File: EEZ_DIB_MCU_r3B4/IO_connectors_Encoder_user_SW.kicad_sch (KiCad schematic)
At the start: 39 parts, among them IC1 TPD4E001DRLR, IC2 74AUP1G74DC.125, IC3 CD74HC4050PWR, SW1 TL1100CF160Q, SW2 PEC16-2215F-S0024, X1 DS1024-2*20R0, X2 DS1013-16SSIB1, X3 691322110005

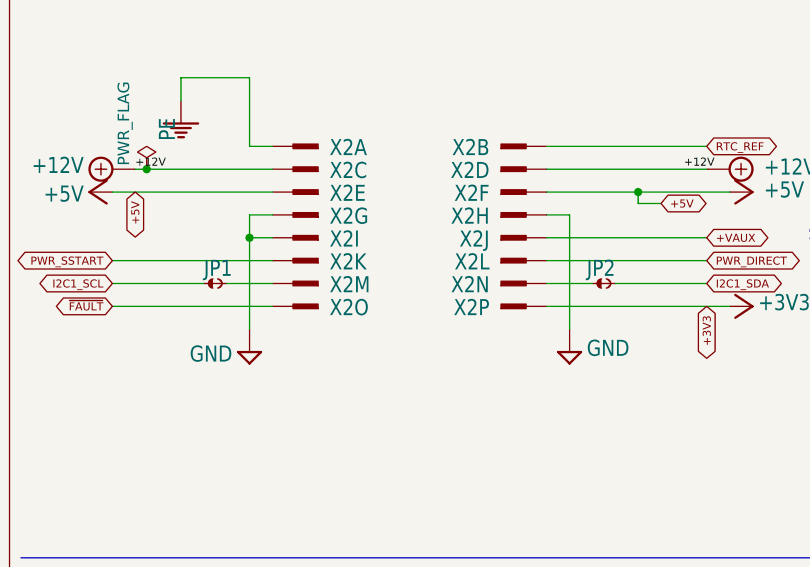
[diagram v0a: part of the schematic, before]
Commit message: Switching MCU to KiCad 7 - moving MCU and SDRAM from board
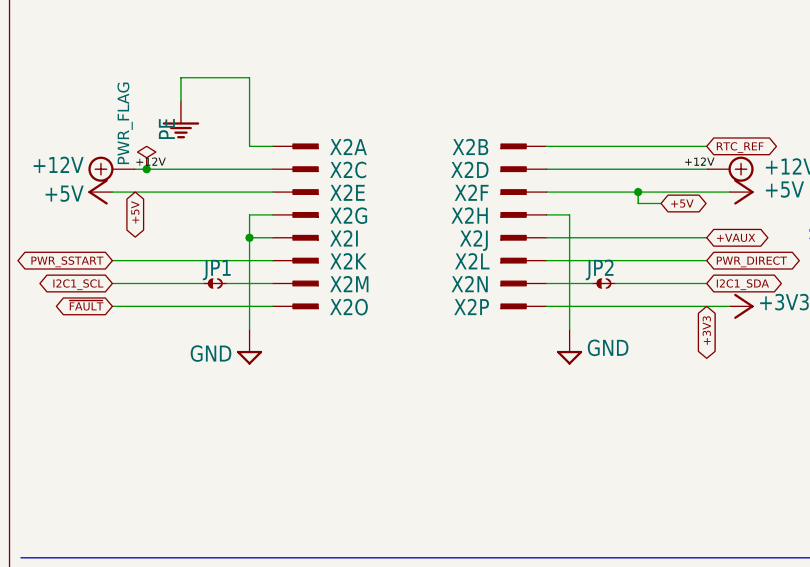
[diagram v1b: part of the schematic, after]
